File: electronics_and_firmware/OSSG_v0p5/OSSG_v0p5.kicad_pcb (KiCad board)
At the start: 4 copper layers, 93 x 10.5 mm, 80 parts, among them J1 Conn_01x05_Male, J2 Ext RGB, J3 USB_B_Micro, J4 Touch, J5 Ext. HUD, Q1 2SC4617R BR, Q2 2SC4617R BR, Q3 PMZ290UNE2YL, Q4 YJQD30P02A, Q5 PMZ350UPEYL, SW1 SW_SPST, SW2 Power, U1 SPH0645LMH, U2 ESP32-PICO-D4, U3 CH9102F, U4 XC61CC3002MR, U5 AP5054HTC, U6 MAX17048, U7 NCP167BMX330TBG, U8 SY7088, U9 LY68L6400SLIT_PSRAM

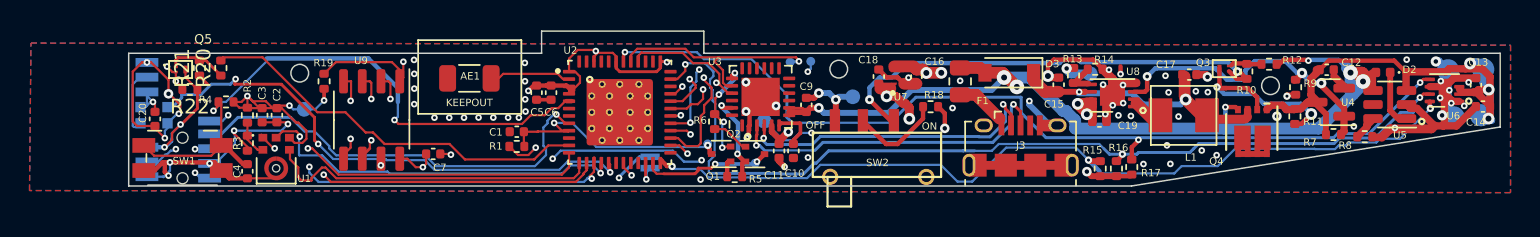
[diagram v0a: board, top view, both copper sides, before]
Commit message: final v0.5 PCB and components order files
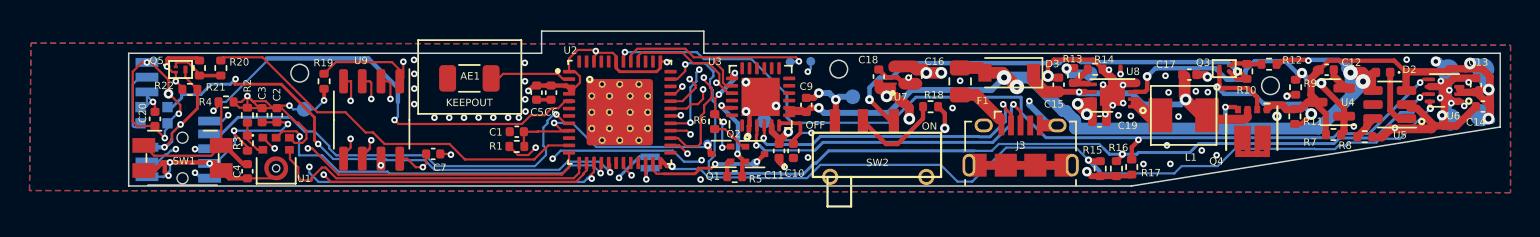
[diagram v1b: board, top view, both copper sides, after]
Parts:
- moved TP17 0.29 mm to (156.6, 79.5)
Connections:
- Q5 pad 1: Net-(R20-Pad1) -> Net-(Q5-Pad1)
- R20 pad 1: Net-(R20-Pad1) -> Net-(Q5-Pad1)
- R21 pad 1: BATT1- -> Net-(Q5-Pad1)
- R21 pad 2: Net-(R20-Pad1) -> +3V3
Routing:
- net Net-(R20-Pad1): track 4.11 -> 0.00 mm
- net Net-(Q5-Pad1): track 0.00 -> 3.79 mm
- net +3V3: track 68.5 -> 71.6 mm
- net BATT1-: track 100.6 -> 99.7 mm
